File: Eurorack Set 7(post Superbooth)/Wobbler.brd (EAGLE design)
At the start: 59.6 x 106.5 mm, 146 parts, among them IC1 LD1117AS33TR, IC3 TL074D, IC4 MCP6004, J1 PJ-341, J12 PJ-341, J13 PJ-341, J14 POWERSMT, J2 PJ-341, J3 PJ-341, J4 PJ-341, J5 PJ-341, J6 PJ-341, J7 PJ-341, J8 PJ-341, Q1 MMBT3904, Q2 MMBT3904, Q3 MMBT3904, Q5 MMBT3904, U1 MKL02Z32VFK4, U2 LM4040DIM3-5.0, U3 74HC595BQ, U4 74HC595BQ, U5 74HC595BQ, U6 24LC16T-I/OT, U7 MCP4822-E/SN

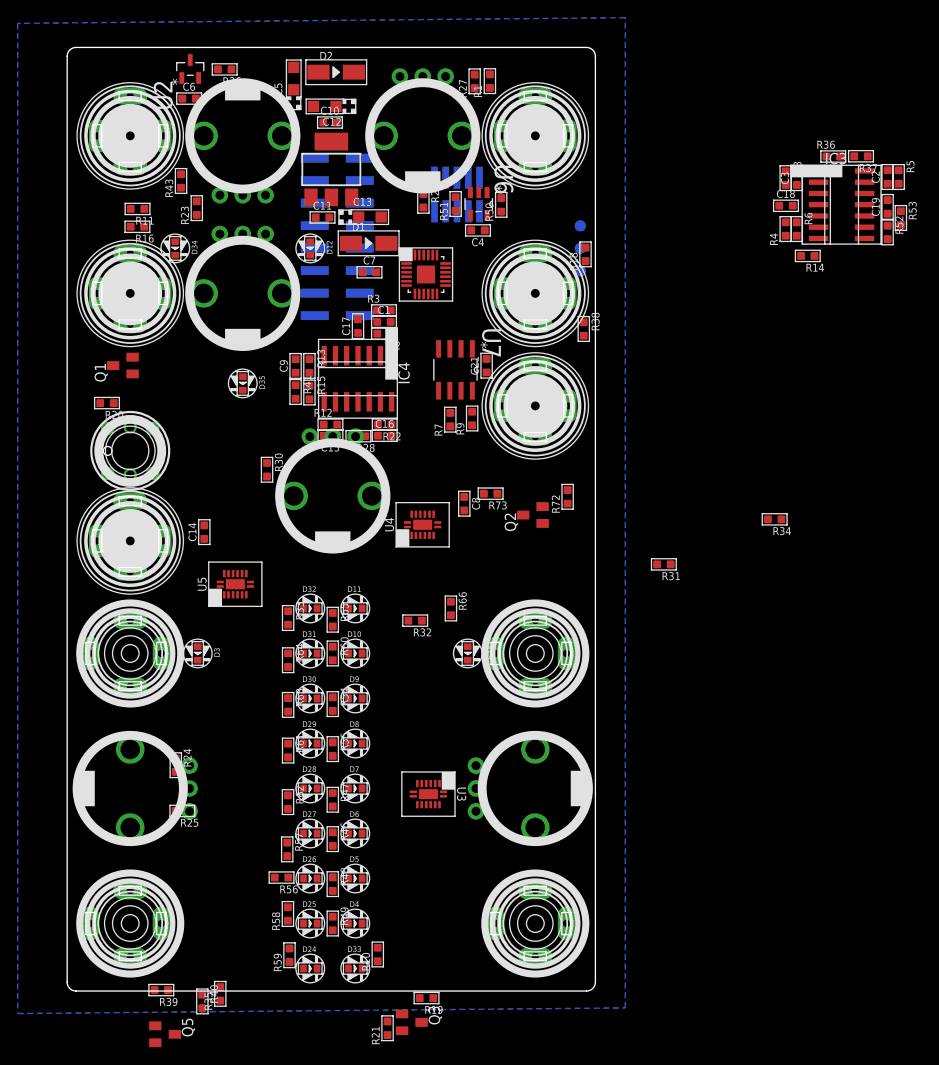
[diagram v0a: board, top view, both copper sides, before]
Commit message: LOTS of updates..... JUNE2017 prototype sprint!
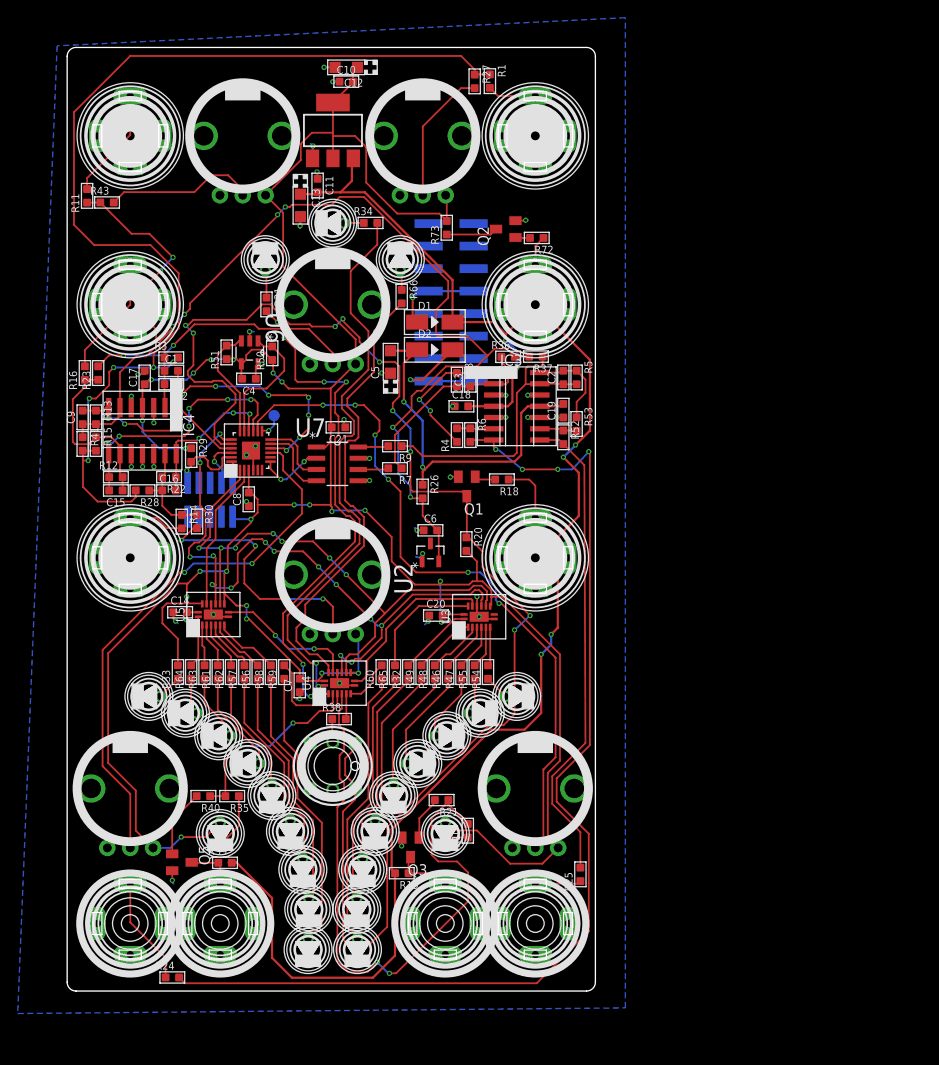
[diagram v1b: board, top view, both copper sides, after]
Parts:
- removed GNDPIN, TX: TPB1,27, testpad:B1,27
- added C20: 100nF, OPL:C0603
- D10, D11, D12, D24, D25, D26, D27, D28, D29, D3, D30, D31, D32, D33, D34, D35, D4, D40, D5, D6, D7, D8, D9: device EurorackModularParts:LED0603 -> EurorackModularParts:3MMLED
- moved R14 76.8 mm to (13.4, 53.0), turned to 270 degrees
- moved U2 60.9 mm to (41.5, 49.5)
- moved R34 56.6 mm to (34.7, 86.7), turned to 0 degrees
- moved C6 55.8 mm to (41.5, 52.0)
- moved R31 53.6 mm to (23.0, 77.5), turned to 270 degrees
- moved R26 52.6 mm to (40.6, 56.4), turned to 270 degrees
- moved R38 52.0 mm to (31.2, 30.7), turned to 0 degrees
- moved J1 48.8 mm to (7.62, 48.9)
- moved C7 47.3 mm to (26.8, 34.5), turned to 90 degrees
- moved J5 45.8 mm to (53.3, 48.9)
- moved R25 45.5 mm to (58.4, 13.2), turned to 90 degrees
- moved SWD1 44.4 mm to (16.6, 55.4), turned to 0 degrees
- moved R4 43.8 mm to (44.5, 62.8)
- moved R20 43.6 mm to (45.6, 50.4), turned to 270 degrees
- moved R6 43.6 mm to (46.0, 62.8)
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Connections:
- removed net N$30 (its old number): R58.2, U5.1
- removed net N$59 (its old number): R60.2, U3.6
- removed net N$63: R66.2, U4.7
- new net N$26: R61.2, U5.3
- new net N$37: R59.2, U4.3
- net 3.3V: now also C20.2
- net ADC_NORMAL: now also U1.9
- net ADC_PHASED: now also U1.14
- net GND: now also C20.1; no longer GNDPIN.TP
- net N$1: now also U5.15; no longer U4.15
- net N$19: now also R64.2, U5.1; no longer R32.2, U4.1
- net N$22: now also R63.2, U5.2; no longer R59.2, U5.15
- net N$31: now also R57.2, U5.5; no longer R56.2, U5.2
- net N$35: now also R56.2, U5.6; no longer R57.2, U5.3
- net N$36: now also R58.2, U5.7; no longer R34.2, U4.3
- net N$38: now also R54.2, U3.7; no longer R61.2, U5.5
- net N$39: now also R55.2, U3.6; no longer R63.2, U5.6
- net N$40: now also R47.2, U3.5; no longer R64.2, U5.7
- net N$43: now also R46.2, U3.4; no longer TX.TP, U1.14
- net N$53: now also R48.2, U3.3; no longer R49.2, U3.15
- net N$54: now also R49.2, U3.2; no longer R48.2, U3.1
- net N$55: now also R32.2, U3.1; no longer R46.2, U3.2
- net N$56: now also R65.2, U3.15; no longer R47.2, U3.3
- net N$57: now also R60.2, U4.7; no longer R55.2, U3.4
- net N$58: now also R34.2, U4.1; no longer R54.2, U3.5
- net N$62: now also R66.2, U4.15; no longer R65.2, U3.7
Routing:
- net 3.3V: track 0.00 -> 327.8 mm, vias 0 -> 24
- net 12V: track 0.00 -> 173.0 mm, vias 0 -> 6
- net RESET_PATTERN: track 0.00 -> 161.5 mm, vias 0 -> 10
- net REF_-5V: track 0.00 -> 132.5 mm, vias 0 -> 11
- net NORMALOUT: track 0.00 -> 122.2 mm, vias 0 -> 4
- net N$8: track 0.00 -> 93.4 mm
- net ADC_PHASED: track 0.00 -> 78.5 mm, vias 0 -> 6
- net LATCH: track 0.00 -> 78.1 mm, vias 0 -> 14
- net OUT_LFOCYCLEMID: track 0.00 -> 69.7 mm, vias 0 -> 2
- net CLOCK: track 0.00 -> 66.4 mm, vias 0 -> 7
- net N$58: track 0.00 -> 64.5 mm, vias 0 -> 2
- net ADC_NORMAL: track 0.00 -> 61.5 mm, vias 0 -> 2
- net GND: track 0.00 -> 61.1 mm, vias 0 -> 39
- net N$59: track 0.00 -> 59.4 mm, vias 0 -> 6
- net PHASEDOUT: track 0.00 -> 54.5 mm
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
